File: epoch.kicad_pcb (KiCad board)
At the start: 4 copper layers, 28 x 34 mm, 29 parts, among them J1 USB_OTG, J2 CONN_01X05, P3 CONN_01X10, SW1 SW_Reset, SW2 SW_Up, SW3 SW_Middle, SW4 SW_Down, U1 MIC5219-3.3BM5, U2 ATSAMD21Ennc-AU, U3 DS3231MZ, U4 MCP7940N-I/SN, U5 74HC1G14GW

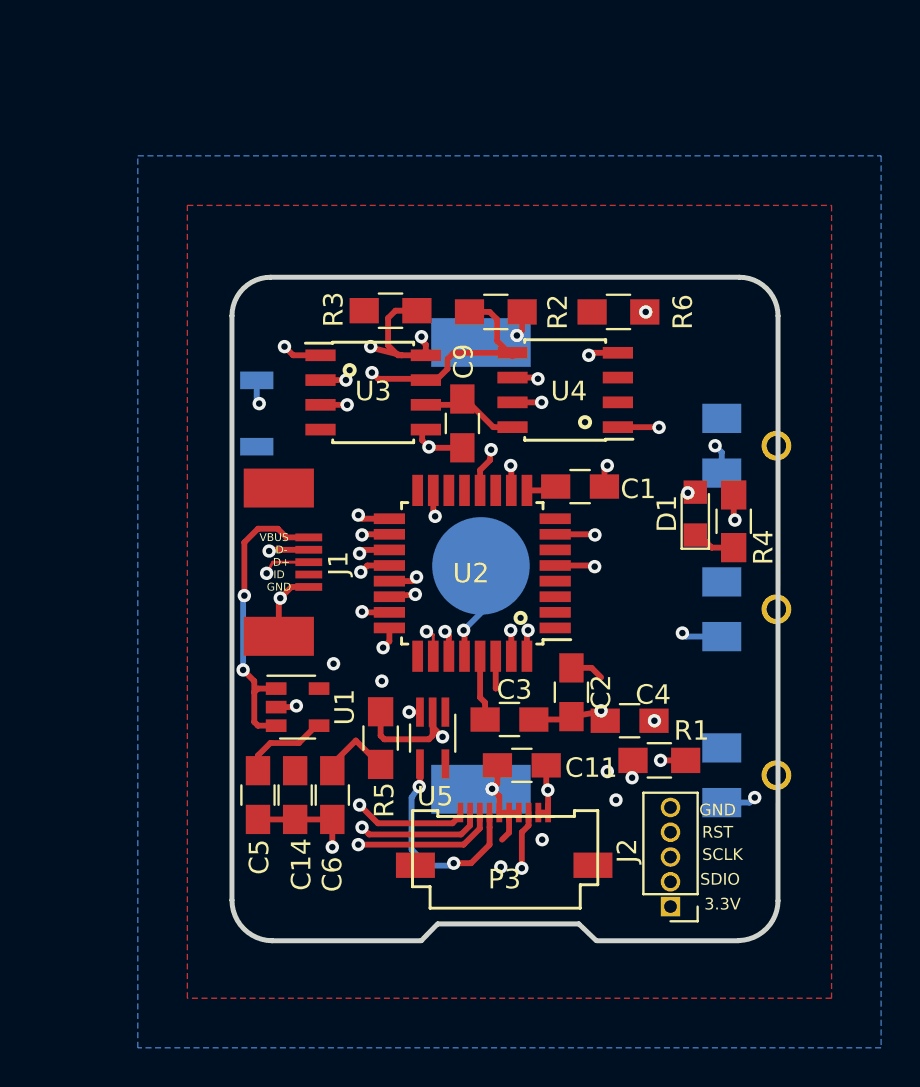
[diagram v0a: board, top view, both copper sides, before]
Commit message: Add drills back to PCB...Note this PCB does not include the battery protection switch which is shown in the schematic.
Not sure I have the PBC space to do this.  Maybe do a separate board.  Not sure.
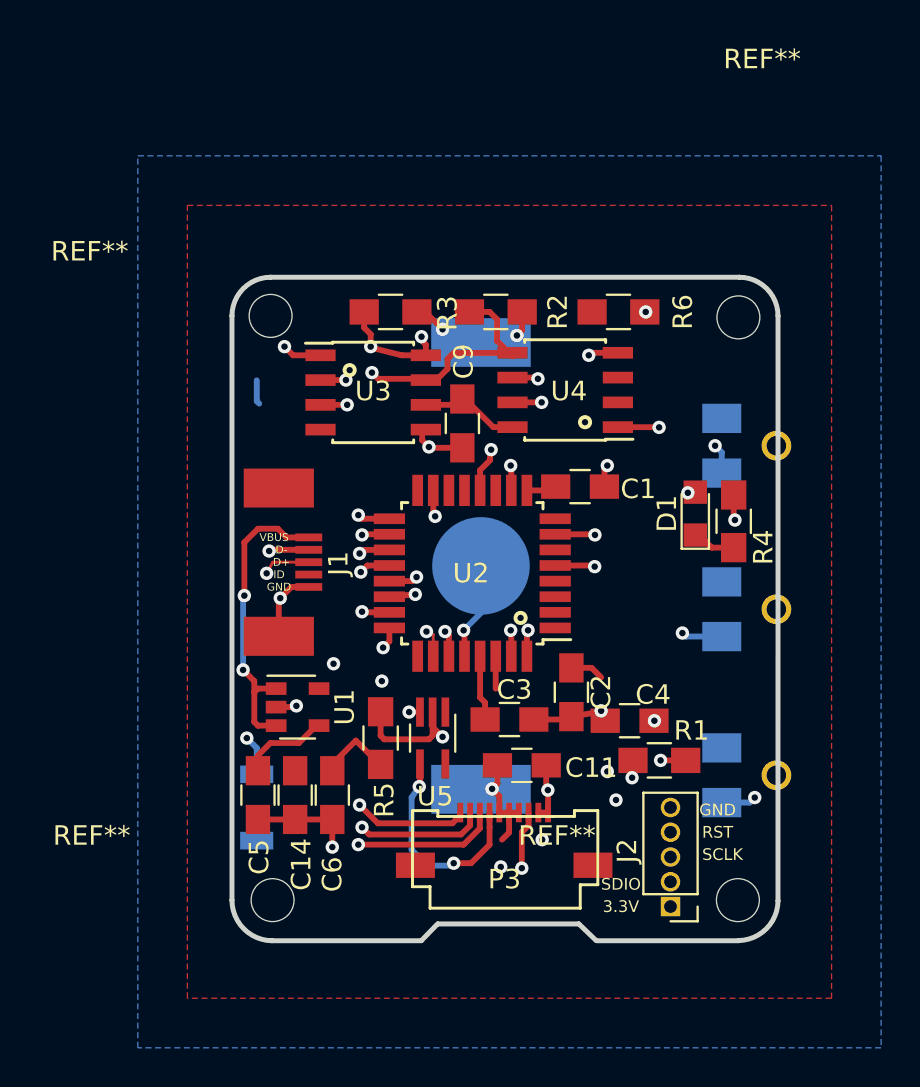
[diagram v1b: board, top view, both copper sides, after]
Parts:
- added REF**: 1pin, Connectors:1pin_nosilk, F.Cu at (103.3, 56.5)
- added REF**: 1pin, Connectors:1pin_nosilk, F.Cu at (127.3, 56.5)
- added REF**: 1pin, Connectors:1pin_nosilk, F.Cu at (103.4, 86.4)
- added REF**: 1pin, Connectors:1pin_nosilk, F.Cu at (127.3, 86.4)
- moved SW1 20.2 mm to (102.6, 81.7)
- moved R3 0.06 mm to (109.5, 56.3), turned to 180 degrees
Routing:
- net Net-(R1-Pad1): track 40.2 -> 27.4 mm
- net (+3.3): track 21.1 -> 25.0 mm, vias 2 -> 3
- net SCL: track 34.0 -> 32.0 mm
- net (no net): track 0.00 -> 1.24 mm

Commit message: Revert "Add drills back to PCB...Note this PCB does not include the battery protection switch which is shown in the schematic."
This reverts commit 0a23e0f0d40f65d1b6f1174f50c74f54a2cdcd00.
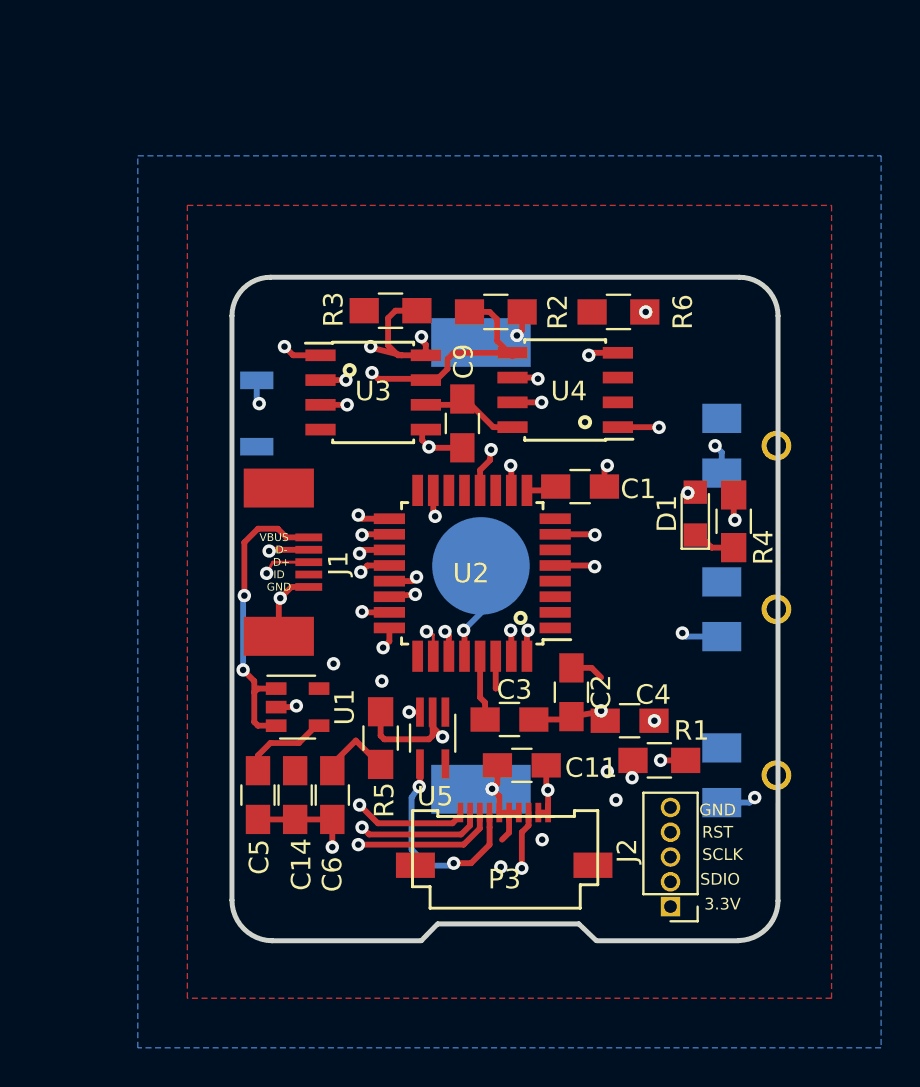
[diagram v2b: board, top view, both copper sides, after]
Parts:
- removed REF** (x4): 1pin, Connectors:1pin_nosilk
- moved SW1 20.2 mm to (102.6, 61.5)
- moved R3 0.06 mm to (109.5, 56.2), turned to 0 degrees
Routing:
- net Net-(R1-Pad1): track 27.4 -> 40.2 mm
- net (+3.3): track 25.0 -> 21.1 mm, vias 3 -> 2
- net SCL: track 32.0 -> 34.0 mm
- net (no net): track 1.24 -> 0.00 mm
